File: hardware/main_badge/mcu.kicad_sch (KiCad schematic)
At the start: 19 parts, among them U1 RP2350B, U2 W25Q128JVS, Y1 12MHz

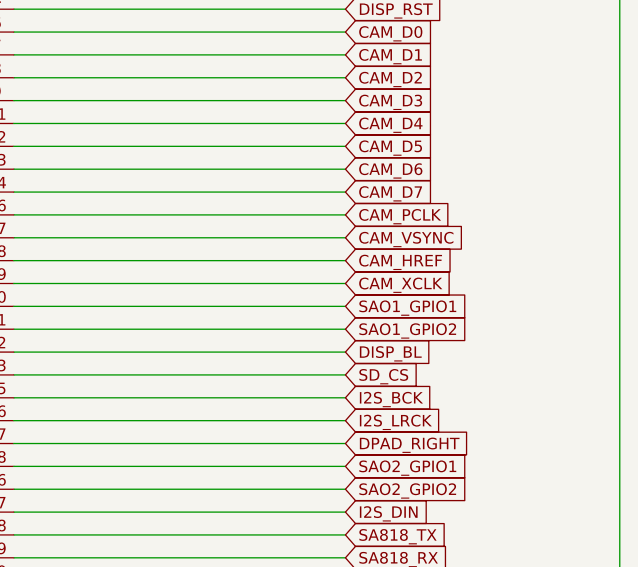
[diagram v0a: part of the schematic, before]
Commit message: main board done except for placing LEDs and drawing ears... I think
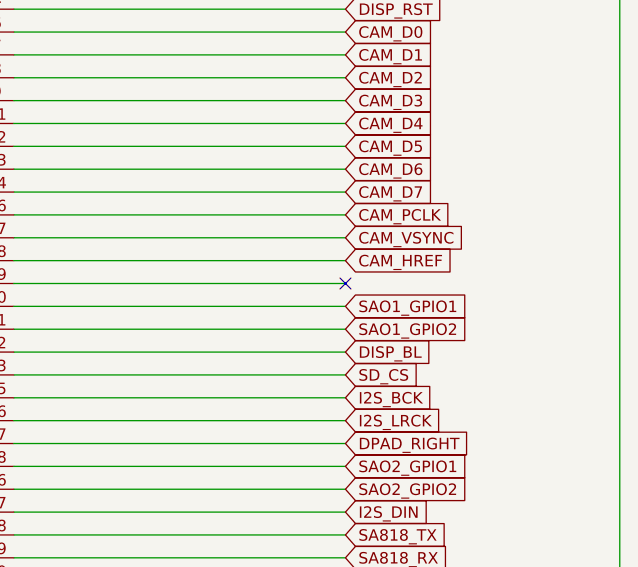
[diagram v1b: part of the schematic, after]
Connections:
- net CAM_XCLK: no longer names the net of U1.19 (GPIO19)
- no-connect marks 0 -> 1
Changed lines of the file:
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@@
 		(color 0 0 0 0)
 	)
+	(no_connect
+		(at 207.01 106.68)
+	)
 	(wire
 		(pts
@@
 			(effects
 				(font
-					(size 1.27 1.27)
-				)
-				(justify left)
-				(hide yes)
-			)
-		)
-	)
-	(global_label "CAM_XCLK"
-		(shape input)
-		(at 207.01 106.68 0)
-		(fields_autoplaced yes)
-		(effects
-			(font
-				(size 1.27 1.27)
-			)
-			(justify left)
-		)
-		(property "Intersheetrefs" "${INTERSHEET_REFS}"
-			(at 219.5504 106.68 0)
-			(effects
-				(font

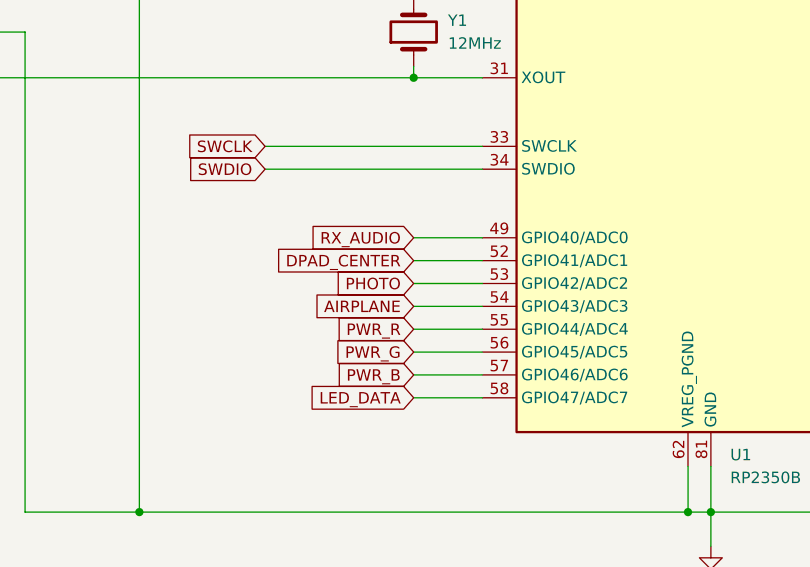
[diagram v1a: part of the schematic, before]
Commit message: screen LEDs placed, photo button removed
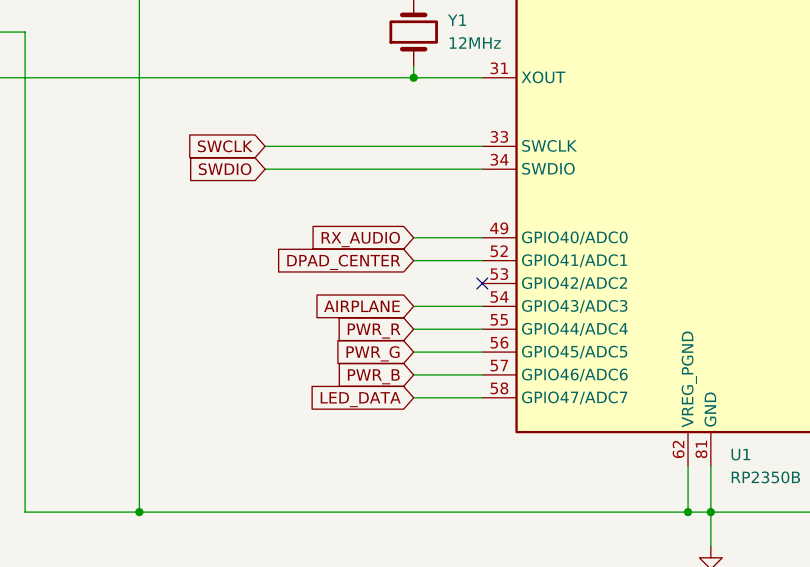
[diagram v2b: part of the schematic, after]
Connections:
- net PHOTO: no longer names the net of U1.53 (GPIO42/ADC2)
- no-connect marks 1 -> 2
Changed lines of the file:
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@@
+	)
+	(no_connect
+		(at 119.38 144.78)
 	)
 	(no_connect
@@
 	(wire
 		(pts
-			(xy 111.76 144.78) (xy 119.38 144.78)
-		)
-		(stroke
-			(width 0)
-			(type default)
-		)
-	)
-	(wire
-		(pts
 			(xy 63.5 35.56) (xy 71.12 35.56)
 		)
@@
 				(hide yes)
 			)
-		)
-	)
-	(global_label "PHOTO"
-		(shape input)
-		(at 111.76 144.78 180)
-		(fields_autoplaced yes)
-		(effects
-			(font
-				(size 1.27 1.27)
-			)
-			(justify right)
-		)
-		(property "Intersheetrefs" "${INTERSHEET_REFS}"
-			(at 102.5457 144.78 0)
-			(effects
-				(font
-					(size 1.27 1.27)
-				)
-				(justify right)
-				(hide yes)
-			)
